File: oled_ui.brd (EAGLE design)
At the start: 84.5 x 19.2 mm, 25 parts, among them IC1 74HC14D

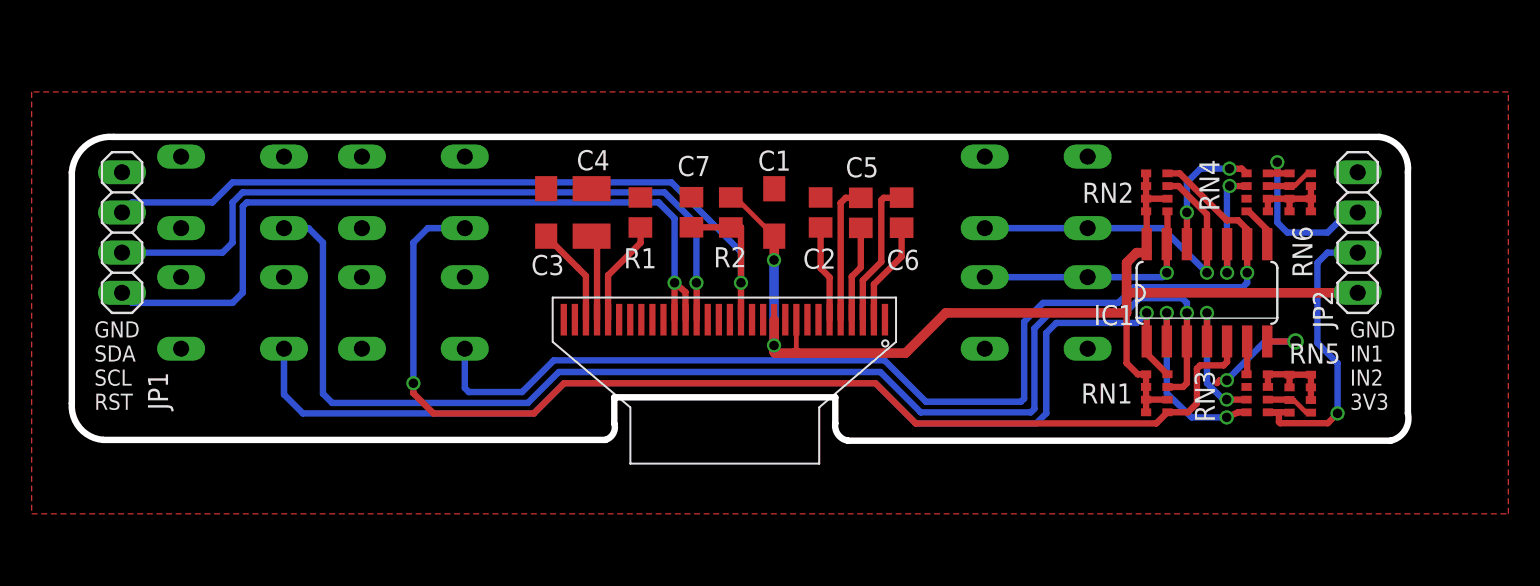
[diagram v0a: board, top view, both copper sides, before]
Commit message: big flip
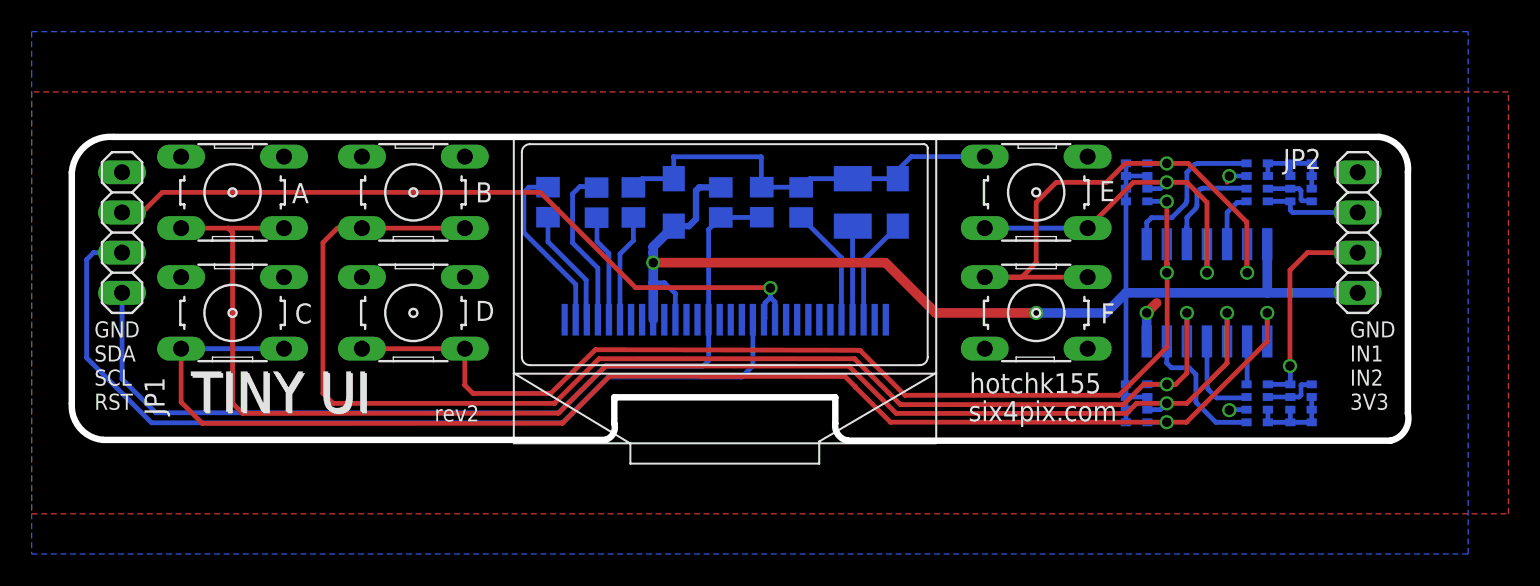
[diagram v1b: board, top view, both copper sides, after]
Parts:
- moved U$1 26.7 mm to (27.9, -5.08), flipped to the top
- moved C6 22.4 mm to (30.1, 17.2), flipped to the bottom, turned to 270 degrees
- moved C3 22.2 mm to (52.2, 17.1), flipped to the bottom
- moved C5 16.7 mm to (33.2, 17.1), flipped to the bottom, turned to 270 degrees
- moved C4 16.5 mm to (49.4, 17.1), flipped to the bottom
- moved C2 11.9 mm to (35.5, 17.1), flipped to the bottom
- moved R1 10.2 mm to (46.1, 17.1), flipped to the bottom
- moved C1 6.38 mm to (38.0, 17.1), flipped to the bottom
- moved C7 4.49 mm to (43.6, 17.2), flipped to the bottom
- moved RN1 1.42 mm to (67.3, 4.45), flipped to the bottom, turned to 270 degrees
- moved RN2 1.42 mm to (67.3, 18.4), flipped to the bottom, turned to 270 degrees
- moved R2 0.90 mm to (41.0, 17.1), flipped to the bottom
- moved RN6 0.64 mm to (77.7, 18.4), flipped to the bottom, turned to 270 degrees
- moved RN3 0.63 mm to (74.9, 4.45), flipped to the bottom, turned to 90 degrees
- moved RN4 0.63 mm to (74.9, 18.4), flipped to the bottom, turned to 90 degrees
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- renumbered S1 to E, S2 to F, S3 to B, S4 to A, S5 to D, S6 to C
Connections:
- net N$11: now also C.1
- net N$12: now also D.1
- net N$5: now also B.1
- net N$9: now also A.1
- net RST: now also JP1.1; no longer JP1.3
- net SDA: now also JP1.3; no longer JP1.1
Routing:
- net GND: track 7.88 -> 32.4 mm, vias 2 -> 3
- net N$14: track 15.5 -> 36.1 mm, vias 1 -> 2
- net N$11: track 70.1 -> 88.5 mm, vias 1 -> 2
- net N$5: track 71.1 -> 84.3 mm, vias 1 -> 2
- net 3V3: track 72.4 -> 84.1 mm
- net SCL: track 46.2 -> 56.9 mm, vias 1 -> 0
- net N$19: track 12.6 -> 2.73 mm, vias 2 -> 0
- net N$9: track 81.6 -> 91.0 mm, vias 1 -> 2
- net N$17: track 2.70 -> 10.3 mm
- net N$20: track 2.09 -> 8.99 mm
- net BUTTONS_OUT2: track 19.6 -> 13.4 mm
- net BUTTONS_OUT1: track 11.8 -> 6.29 mm, vias 1 -> 0
- net N$15: track 8.16 -> 3.53 mm, vias 2 -> 0
- net N$2: track 6.54 -> 11.1 mm
- net N$3: track 6.04 -> 10.4 mm
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- added copper zone on layer 16, net GND
